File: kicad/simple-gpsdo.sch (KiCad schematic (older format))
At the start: 93 parts, among them J2 PWR, J3 ISP, J4 GPS_NEO, J5 GPS_IN, J6 10MHz_OUT, J7 NEO-6M, J8 10MHz_OUT, J9 USB_C_Receptacle_USB2.0, SW1 RST, U1 BD50FC0FP-E2, U2 ATmega32U4-AU, U3 MC74HC390, U4 CD74HC4046AM96, U5 BD50FC0FP-E2, U6 LM7171, U7 LM7171, U8 LM35-D, U9 AP62301WU-7, Y1 16MHz, Y2 NV47X

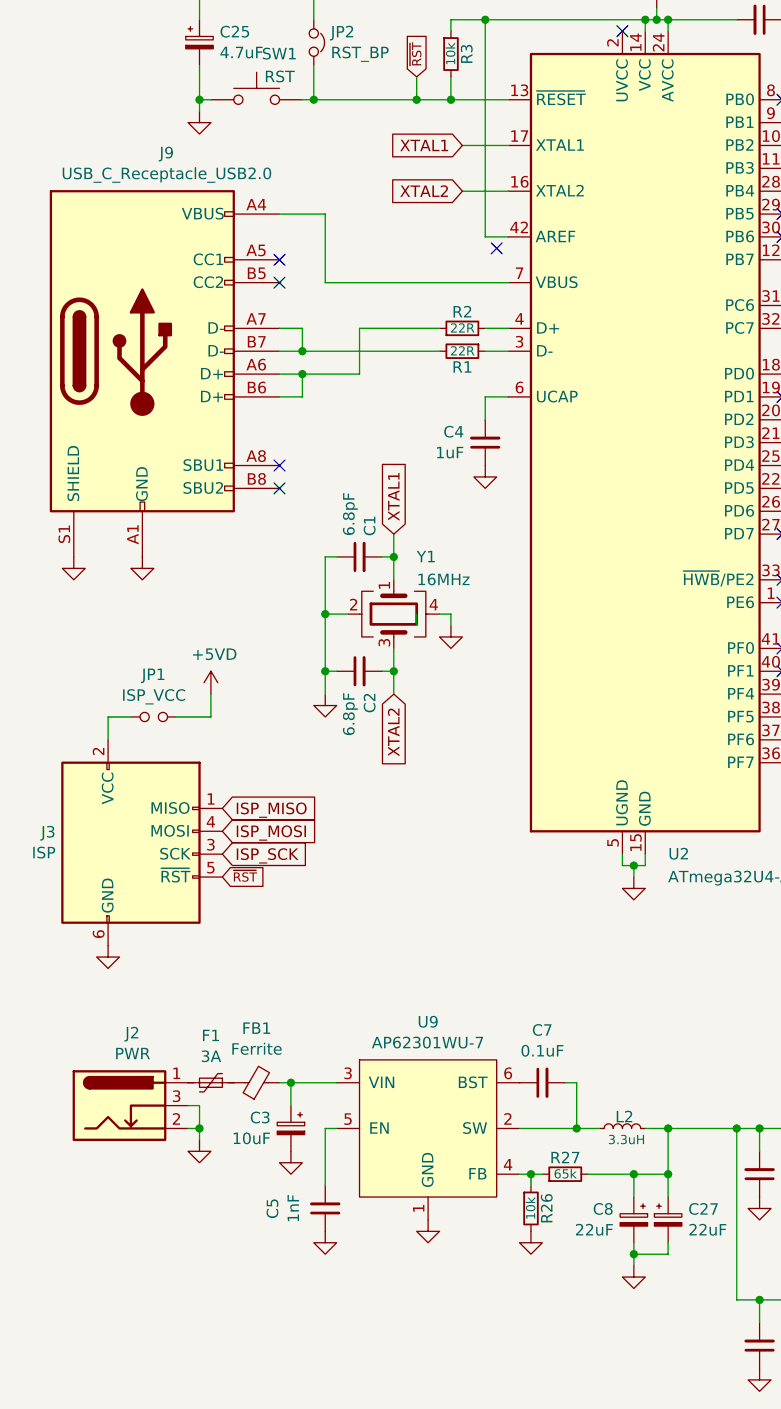
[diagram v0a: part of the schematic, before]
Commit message: finalizing schematic
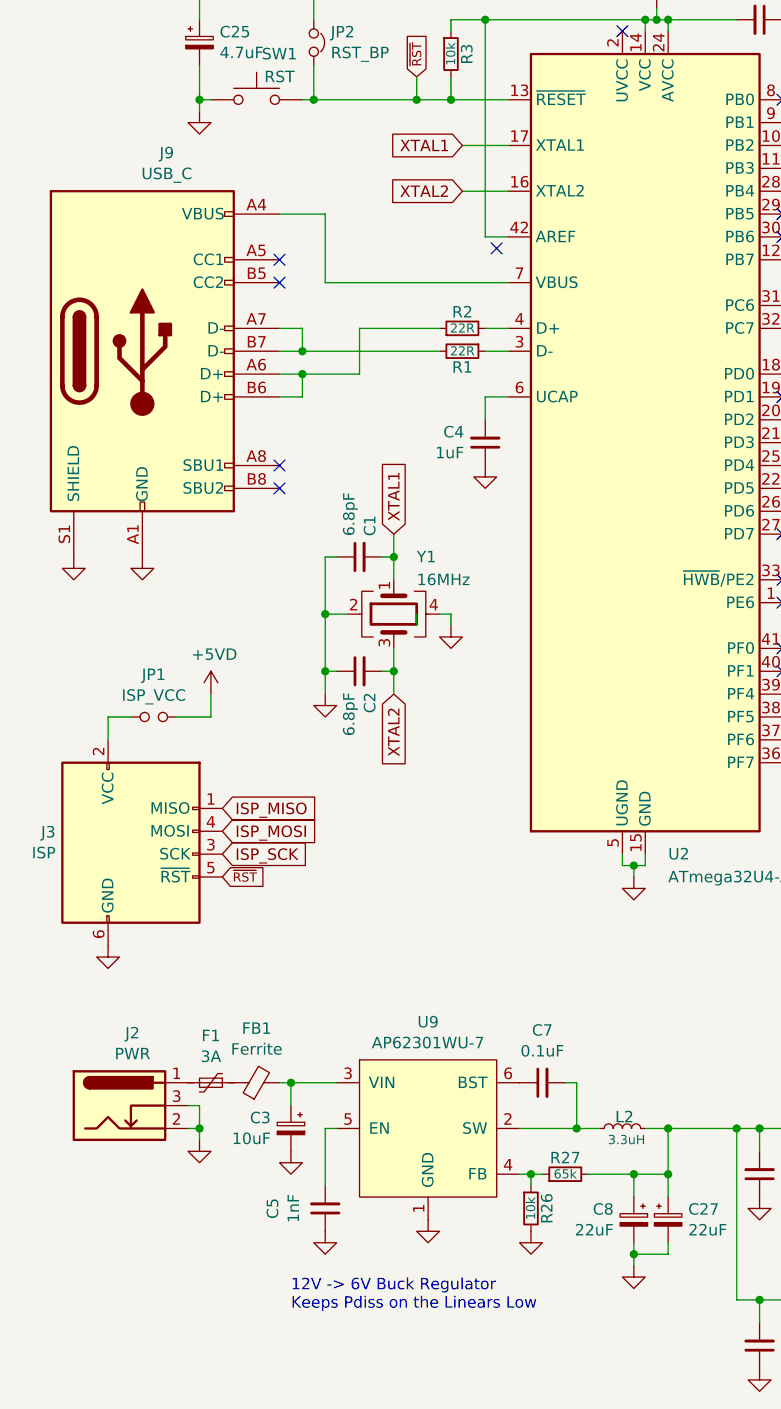
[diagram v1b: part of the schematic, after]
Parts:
- J9: value USB_C_Receptacle_USB2.0 -> USB_C
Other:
- note added: "12V -> 6V Buck Regulator\nKeeps Pdiss on the Linears Low"
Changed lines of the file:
@@
 P 1300 3100
 F 0 "J9" H 1407 3967 50  0000 C CNN
-F 1 "USB_C_Receptacle_USB2.0" H 1407 3876 50  0000 C CNN
+F 1 "USB_C" H 1407 3876 50  0000 C CNN
 F 2 "Kycon:KUSBX-SL-CS1N14-B" H 1450 3100 50  0001 C CNN
 F 3 "https://www.usb.org/sites/default/files/documents/usb_type-c.zip" H 1450 3100 50  0001 C CNN
@@
 Connection ~ 3600 6500
 Connection ~ 3900 6500
+Text Notes 1950 7300 0    50   ~ 0
+12V -> 6V Buck Regulator\nKeeps Pdiss on the Linears Low
 $EndSCHEMATC
